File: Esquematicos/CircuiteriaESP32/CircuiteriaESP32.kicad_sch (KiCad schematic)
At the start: 11 parts, among them J1 Conn_01x19, J2 Conn_01x19

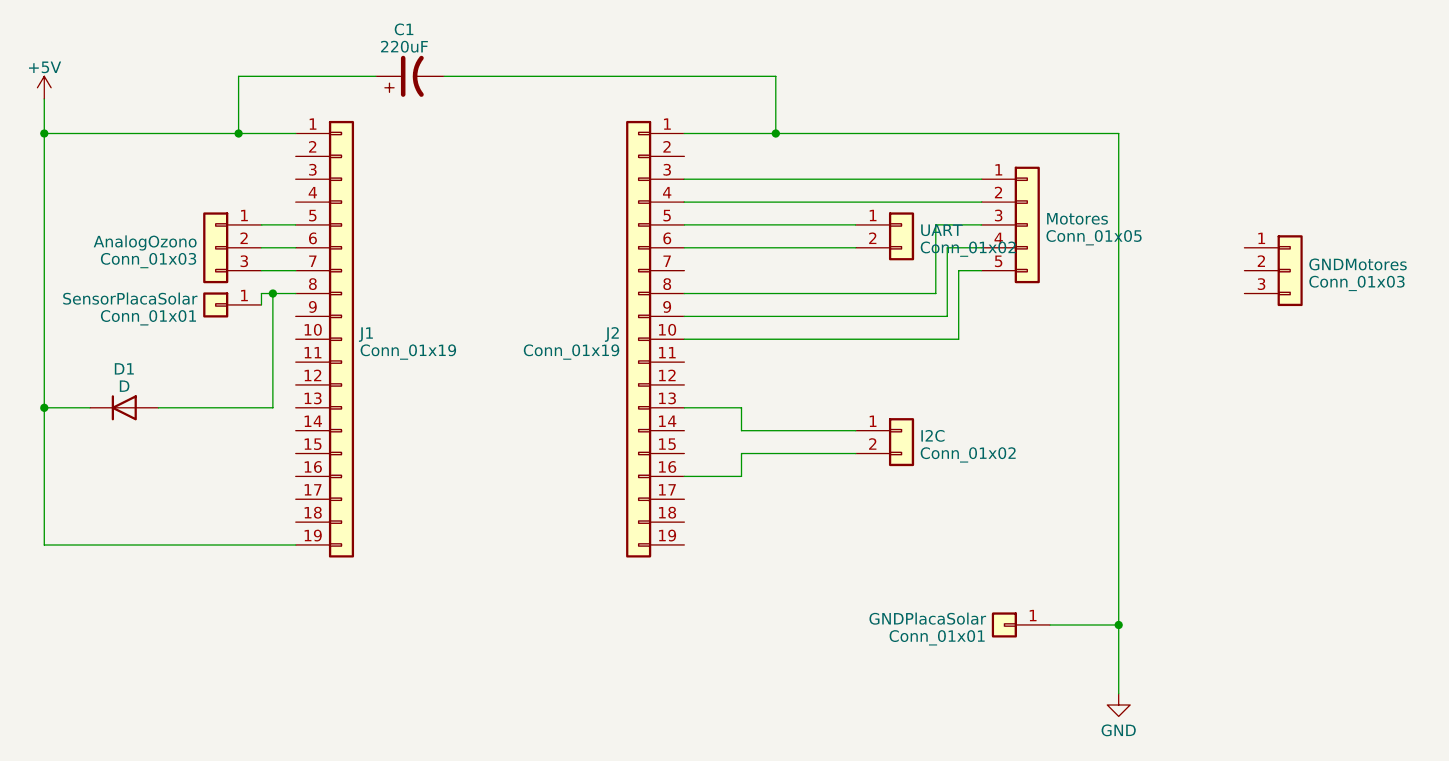
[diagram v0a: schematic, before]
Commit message: Ajustadas algunas cosas, to-do
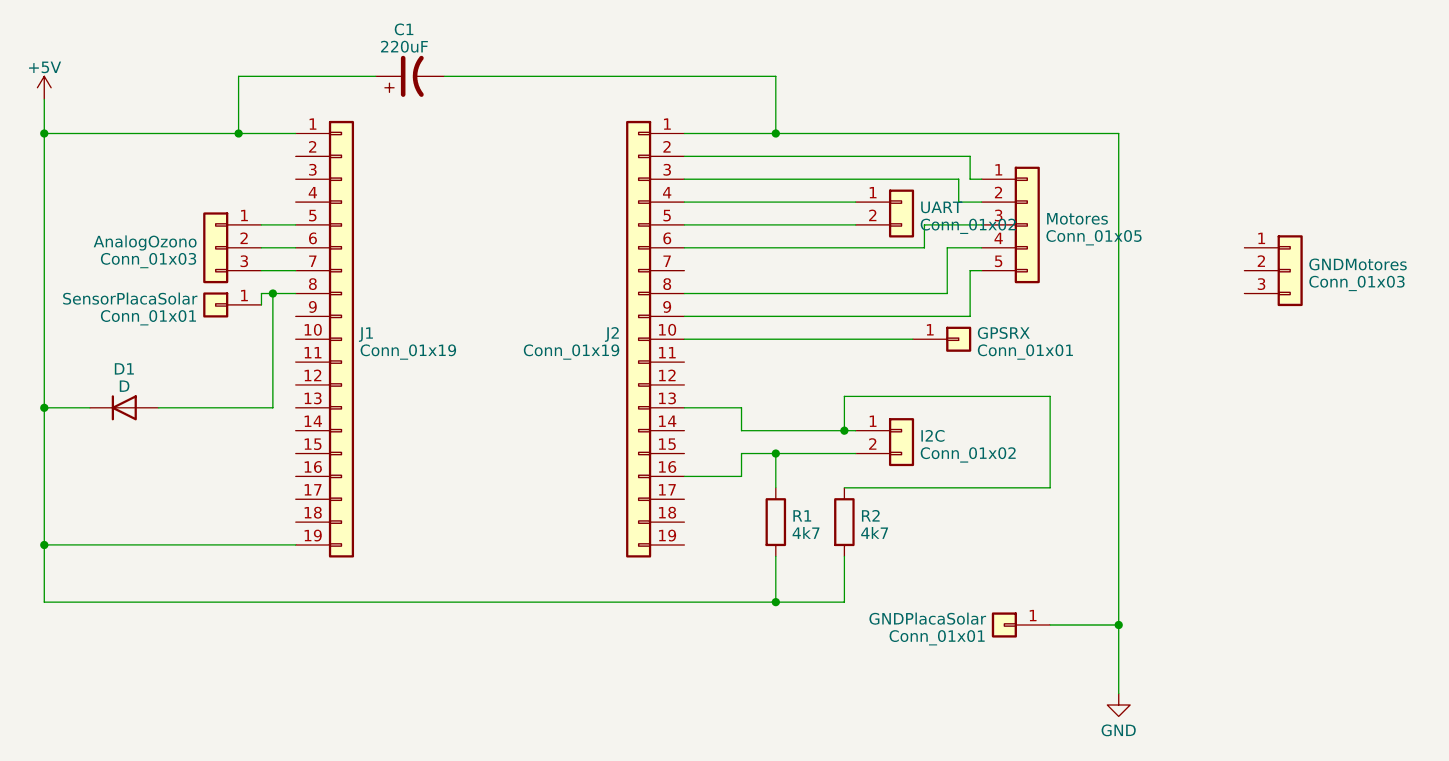
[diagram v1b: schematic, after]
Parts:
- added GPSRX: Conn_01x01, symbol Connector_Generic:Conn_01x01
- added R1, R2: 4k7, symbol Device:R
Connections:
- net +5V: now also R1.2, R2.2
- net at I2C.1 (Pin_1), J2.13 (Pin_13): now also R2.1
- net at I2C.2 (Pin_2), J2.16 (Pin_16): now also R1.1
- net at Motores.1 (Pin_1): now also J2.2 (Pin_2); no longer J2.3 (Pin_3)
- net at Motores.2 (Pin_2): now also J2.3 (Pin_3); no longer J2.4 (Pin_4)
- net at Motores.3 (Pin_3): now also J2.6 (Pin_6); no longer J2.8 (Pin_8)
- net at Motores.4 (Pin_4): now also J2.8 (Pin_8); no longer J2.9 (Pin_9)
- net at J2.10 (Pin_10): now also GPSRX.1 (Pin_1); no longer Motores.5 (Pin_5)
- net at UART.1 (Pin_1): now also J2.4 (Pin_4); no longer J2.5 (Pin_5)
- net at UART.2 (Pin_2): now also J2.5 (Pin_5); no longer J2.6 (Pin_6)
- new net: J2.9 (Pin_9), Motores.5 (Pin_5)
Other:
- moved on the sheet: UART
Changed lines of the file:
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@@
 (kicad_sch (version 20230121) (generator eeschema)
   (paper "A4")
+  (junction (at 146.05 97.79) (diameter 0) (color 0 0 0 0)
+  )
+  (junction (at 146.05 81.28) (diameter 0) (color 0 0 0 0)
+  )
   (junction (at 64.77 76.2) (diameter 0) (color 0 0 0 0)
   )
   (junction (at 86.36 45.72) (diameter 0) (color 0 0 0 0)
   )
+  (junction (at 153.67 78.74) (diameter 0) (color 0 0 0 0)
+  )
   (junction (at 184.15 100.33) (diameter 0) (color 0 0 0 0)
   )
@@
   (junction (at 90.17 63.5) (diameter 0) (color 0 0 0 0)
   )
-  (wire (pts (xy 168.91 60.96) (xy 166.37 60.96))
-    (stroke (width 0) (type default))
+  (junction (at 64.77 91.44) (diameter 0) (color 0 0 0 0)
   )
   (wire (pts (xy 64.77 91.44) (xy 64.77 76.2))
@@
     (stroke (width 0) (type default))
   )
-  (wire (pts (xy 135.89 58.42) (xy 154.94 58.42))
+  (wire (pts (xy 165.1 58.42) (xy 165.1 63.5))
+    (stroke (width 0) (type default))
+  )
+  (wire (pts (xy 153.67 78.74) (xy 142.24 78.74))
+    (stroke (width 0) (type default))
+  )
+  (wire (pts (xy 146.05 92.71) (xy 146.05 97.79))
     (stroke (width 0) (type default))
   )
@@
     (stroke (width 0) (type default))
   )
-  (wire (pts (xy 163.83 63.5) (xy 135.89 63.5))
-    (stroke (width 0) (type default))
-  )
   (wire (pts (xy 64.77 76.2) (xy 69.85 76.2))
     (stroke (width 0) (type default))
   )
-  (wire (pts (xy 168.91 55.88) (xy 163.83 55.88))
+  (wire (pts (xy 135.89 66.04) (xy 167.64 66.04))
     (stroke (width 0) (type default))
   )
@@
     (stroke (width 0) (type default))
   )
-  (wire (pts (xy 135.89 50.8) (xy 168.91 50.8))
-    (stroke (width 0) (type default))
-  )
   (wire (pts (xy 90.17 63.5) (xy 88.9 63.5))
     (stroke (width 0) (type default))
   )
+  (wire (pts (xy 135.89 55.88) (xy 154.94 55.88))
+    (stroke (width 0) (type default))
+  )
+  (wire (pts (xy 176.53 74.93) (xy 153.67 74.93))
+    (stroke (width 0) (type default))
+  )
   (wire (pts (xy 86.36 45.72) (xy 92.71 45.72))
     (stroke (width 0) (type default))
@@
     (stroke (width 0) (type default))
   )
+  (wire (pts (xy 162.56 58.42) (xy 135.89 58.42))
+    (stroke (width 0) (type default))
+  )
+  (wire (pts (xy 168.91 58.42) (xy 165.1 58.42))
+    (stroke (width 0) (type default))
+  )
+  (wire (pts (xy 153.67 85.09) (xy 176.53 85.09))
+    (stroke (width 0) (type default))
+  )
   (wire (pts (xy 64.77 76.2) (xy 64.77 45.72))
     (stroke (width 0) (type default))
   )
-  (wire (pts (xy 168.91 58.42) (xy 165.1 58.42))
-    (stroke (width 0) (type default))
-  )
   (wire (pts (xy 135.89 45.72) (xy 146.05 45.72))
     (stroke (width 0) (type default))
@@
     (stroke (width 0) (type default))
   )
+  (wire (pts (xy 168.91 53.34) (xy 166.37 53.34))
+    (stroke (width 0) (type default))
+  )
   (wire (pts (xy 88.9 63.5) (xy 88.9 64.77))
     (stroke (width 0) (type default))
   )
-  (wire (pts (xy 165.1 58.42) (xy 165.1 66.04))
+  (wire (pts (xy 135.89 53.34) (xy 154.94 53.34))
+    (stroke (width 0) (type default))
+  )
+  (wire (pts (xy 176.53 85.09) (xy 176.53 74.93))
     (stroke (width 0) (type default))
   )
@@
     (stroke (width 0) (type default))
   )
-  (wire (pts (xy 166.37 60.96) (xy 166.37 68.58))
+  (wire (pts (xy 168.91 50.8) (xy 167.64 50.8))
     (stroke (width 0) (type default))
   )
@@
     (stroke (width 0) (type default))
   )
-  (wire (pts (xy 166.37 68.58) (xy 135.89 68.58))
-    (stroke (width 0) (type default))
-  )
-  (wire (pts (xy 135.89 55.88) (xy 154.94 55.88))
-    (stroke (width 0) (type default))
-  )
-  (wire (pts (xy 154.94 81.28) (xy 142.24 81.28))
+  (wire (pts (xy 154.94 81.28) (xy 146.05 81.28))
     (stroke (width 0) (type default))
   )
@@
     (stroke (width 0) (type default))
   )
+  (wire (pts (xy 167.64 60.96) (xy 167.64 66.04))
+    (stroke (width 0) (type default))
+  )
+  (wire (pts (xy 146.05 97.79) (xy 64.77 97.79))
+    (stroke (width 0) (type default))
+  )
   (wire (pts (xy 90.17 76.2) (xy 90.17 63.5))
     (stroke (width 0) (type default))
   )
-  (wire (pts (xy 154.94 78.74) (xy 142.24 78.74))
+  (wire (pts (xy 154.94 78.74) (xy 153.67 78.74))
     (stroke (width 0) (type default))
   )
@@
     (stroke (width 0) (type default))
   )
+  (wire (pts (xy 167.64 50.8) (xy 167.64 48.26))
+    (stroke (width 0) (type default))
+  )
+  (wire (pts (xy 162.56 55.88) (xy 162.56 58.42))
+    (stroke (width 0) (type default))
+  )
   (wire (pts (xy 64.77 41.91) (xy 64.77 45.72))
     (stroke (width 0) (type default))
   )
+  (wire (pts (xy 146.05 81.28) (xy 146.05 85.09))
+    (stroke (width 0) (type default))
+  )
   (wire (pts (xy 146.05 39.37) (xy 146.05 45.72))
     (stroke (width 0) (type default))
   )
+  (wire (pts (xy 146.05 81.28) (xy 142.24 81.28))
+    (stroke (width 0) (type default))
+  )
+  (wire (pts (xy 153.67 74.93) (xy 153.67 78.74))
+    (stroke (width 0) (type default))
+  )
+  (wire (pts (xy 168.91 60.96) (xy 167.64 60.96))
+    (stroke (width 0) (type default))
+  )
+  (wire (pts (xy 153.67 92.71) (xy 153.67 97.79))
+    (stroke (width 0) (type default))
+  )
   (wire (pts (xy 146.05 45.72) (xy 184.15 45.72))
     (stroke (width 0) (type default))
@@
     (stroke (width 0) (type default))
   )
-  (wire (pts (xy 135.89 53.34) (xy 168.91 53.34))
-    (stroke (width 0) (type default))
-  )
-  (wire (pts (xy 165.1 66.04) (xy 135.89 66.04))
+  (wire (pts (xy 153.67 97.79) (xy 146.05 97.79))
+    (stroke (width 0) (type default))
+  )
+  (wire (pts (xy 166.37 53.34) (xy 166.37 50.8))
+    (stroke (width 0) (type default))
+  )
+  (wire (pts (xy 167.64 48.26) (xy 135.89 48.26))
     (stroke (width 0) (type default))
   )
@@
     (stroke (width 0) (type default))
   )
-  (wire (pts (xy 163.83 55.88) (xy 163.83 63.5))
+  (wire (pts (xy 166.37 50.8) (xy 135.89 50.8))
+    (stroke (width 0) (type default))
+  )
+  (wire (pts (xy 168.91 55.88) (xy 162.56 55.88))
     (stroke (width 0) (type default))
   )
@@
   )
   (wire (pts (xy 86.36 39.37) (xy 86.36 45.72))
+    (stroke (width 0) (type default))
+  )
+  (wire (pts (xy 64.77 97.79) (xy 64.77 91.44))
+    (stroke (width 0) (type default))
+  )
+  (wire (pts (xy 135.89 68.58) (xy 161.29 68.58))
+    (stroke (width 0) (type default))
+  )
+  (wire (pts (xy 165.1 63.5) (xy 135.89 63.5))
     (stroke (width 0) (type default))
   )
@@
     )
   )
+  (symbol (lib_id "Connector_Generic:Conn_01x01") (at 166.37 68.58 0) (unit 1)
+    (in_bom yes) (on_board yes) (dnp no)
+    (property "Reference" "GPSRX" (at 168.402 67.9363 0)
+      (effects (font (size 1.27 1.27)) (justify left))
+    )
+    (property "Value" "Conn_01x01" (at 168.402 69.8573 0)
+      (effects (font (size 1.27 1.27)) (justify left))
+    )
+    (property "Footprint" "" (at 166.37 68.58 0)
+      (effects (font (size 1.27 1.27)) hide)
+    )
+    (property "Datasheet" "~" (at 166.37 68.58 0)
+      (effects (font (size 1.27 1.27)) hide)
+    )
+    (pin "1")
+    (instances
+      (project "CircuiteriaESP32"
+        (path "/916eeabf-7d1d-4f94-90a9-b50ef7656e3c"
+          (reference "GPSRX") (unit 1)
+        )
+      )
+    )
+  )
   (symbol (lib_id "Device:D") (at 73.66 76.2 0) (unit 1)
     (in_bom yes) (on_board yes) (dnp no) (fields_autoplaced)
@@
         (path "/916eeabf-7d1d-4f94-90a9-b50ef7656e3c"
           (reference "#PWR02") (unit 1)
+        )
+      )
+    )
+  )
+  (symbol (lib_id "Device:R") (at 146.05 88.9 0) (unit 1)
+    (in_bom yes) (on_board yes) (dnp no) (fields_autoplaced)
+    (property "Reference" "R1" (at 147.828 88.2563 0)
+      (effects (font (size 1.27 1.27)) (justify left))
+    )
+    (property "Value" "4k7" (at 147.828 90.1773 0)
+      (effects (font (size 1.27 1.27)) (justify left))
+    )
+    (property "Footprint" "" (at 144.272 88.9 90)
+      (effects (font (size 1.27 1.27)) hide)
+    )
+    (property "Datasheet" "~" (at 146.05 88.9 0)
+      (effects (font (size 1.27 1.27)) hide)
+    )
+    (pin "1")
+    (pin "2")
+    (instances
+      (project "CircuiteriaESP32"
+        (path "/916eeabf-7d1d-4f94-90a9-b50ef7656e3c"
+          (reference "R1") (unit 1)
         )
       )
@@
     )
   )
-  (symbol (lib_id "Connector_Generic:Conn_01x02") (at 160.02 55.88 0) (unit 1)
-    (in_bom yes) (on_board yes) (dnp no) (fields_autoplaced)
-    (property "Reference" "UART" (at 162.052 56.5063 0)
-      (effects (font (size 1.27 1.27)) (justify left))
-    )
-    (property "Value" "Conn_01x02" (at 162.052 58.4273 0)
-      (effects (font (size 1.27 1.27)) (justify left))
-    )
-    (property "Footprint" "" (at 160.02 55.88 0)
-      (effects (font (size 1.27 1.27)) hide)
-    )
-    (property "Datasheet" "~" (at 160.02 55.88 0)
+  (symbol (lib_id "Connector_Generic:Conn_01x02") (at 160.02 53.34 0) (unit 1)
+    (in_bom yes) (on_board yes) (dnp no) (fields_autoplaced)
+    (property "Reference" "UART" (at 162.052 53.9663 0)
+      (effects (font (size 1.27 1.27)) (justify left))
+    )
+    (property "Value" "Conn_01x02" (at 162.052 55.8873 0)
+      (effects (font (size 1.27 1.27)) (justify left))
+    )
+    (property "Footprint" "" (at 160.02 53.34 0)
+      (effects (font (size 1.27 1.27)) hide)
+    )
+    (property "Datasheet" "~" (at 160.02 53.34 0)
       (effects (font (size 1.27 1.27)) hide)
     )
@@
         )
       )
+    )
+  )
+  (symbol (lib_id "Device:R") (at 153.67 88.9 0) (unit 1)
+    (in_bom yes) (on_board yes) (dnp no) (fields_autoplaced)
+    (property "Reference" "R2" (at 155.448 88.2563 0)
+      (effects (font (size 1.27 1.27)) (justify left))
+    )
+    (property "Value" "4k7" (at 155.448 90.1773 0)
+      (effects (font (size 1.27 1.27)) (justify left))
+    )
+    (property "Footprint" "" (at 151.892 88.9 90)
+      (effects (font (size 1.27 1.27)) hide)
+    )
+    (property "Datasheet" "~" (at 153.67 88.9 0)
+      (effects (font (size 1.27 1.27)) hide)
+    )
+    (pin "1")
+    (pin "2")
+    (instances
+      (project "CircuiteriaESP32"
+        (path "/916eeabf-7d1d-4f94-90a9-b50ef7656e3c"
+          (reference "R2") (unit 1)
+        )
+      )
